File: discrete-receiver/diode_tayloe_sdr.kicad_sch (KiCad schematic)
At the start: 13 parts, among them J5 Display Connector, X1 YC24.576MUBCE2O

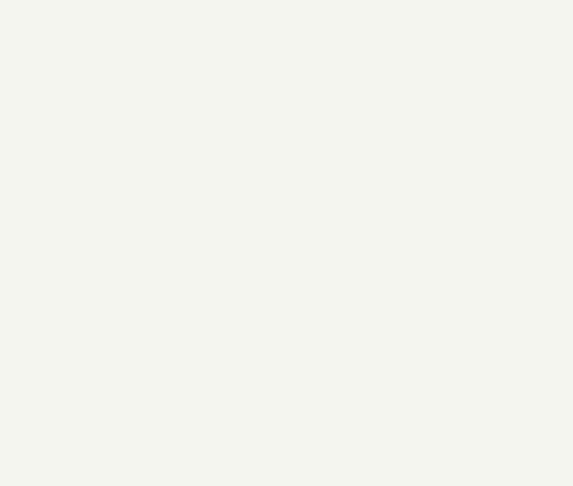
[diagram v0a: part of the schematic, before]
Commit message: PCB Progress
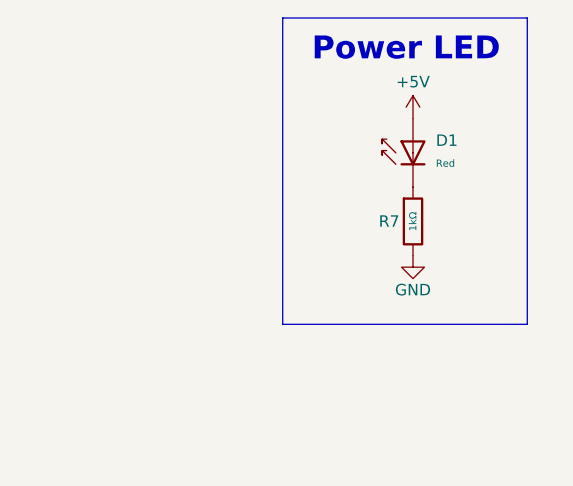
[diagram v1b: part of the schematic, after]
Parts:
- added D1: Red, PCM_JLCPCB:D_0603, symbol PCM_JLCPCB-Diodes:LED,0603,Red
- added R7: 1kΩ, PCM_JLCPCB:R_0402, symbol PCM_JLCPCB-Resistors:0402,1kΩ
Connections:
- net GND: now also R7.2
- new net: D1.1, R7.1
- new net +5V: D1.2
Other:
- note added: "Power LED"
